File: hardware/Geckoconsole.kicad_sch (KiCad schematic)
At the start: 61 parts, among them J1 Conn_01x08_Male, J11 Conn_01x06_Male, J31 Conn_01x07_Female, J50 USB-C, J51 Conn_01x06_Male, J70 I²C, J81 Conn_01x07, Q51 S8050, Q52 S8050, SW2 Reset, SW41 Rotary_Encoder_Switch, U1 ESP32-WROOM-32, U101 AMS1117-3.3, U2 CP2102

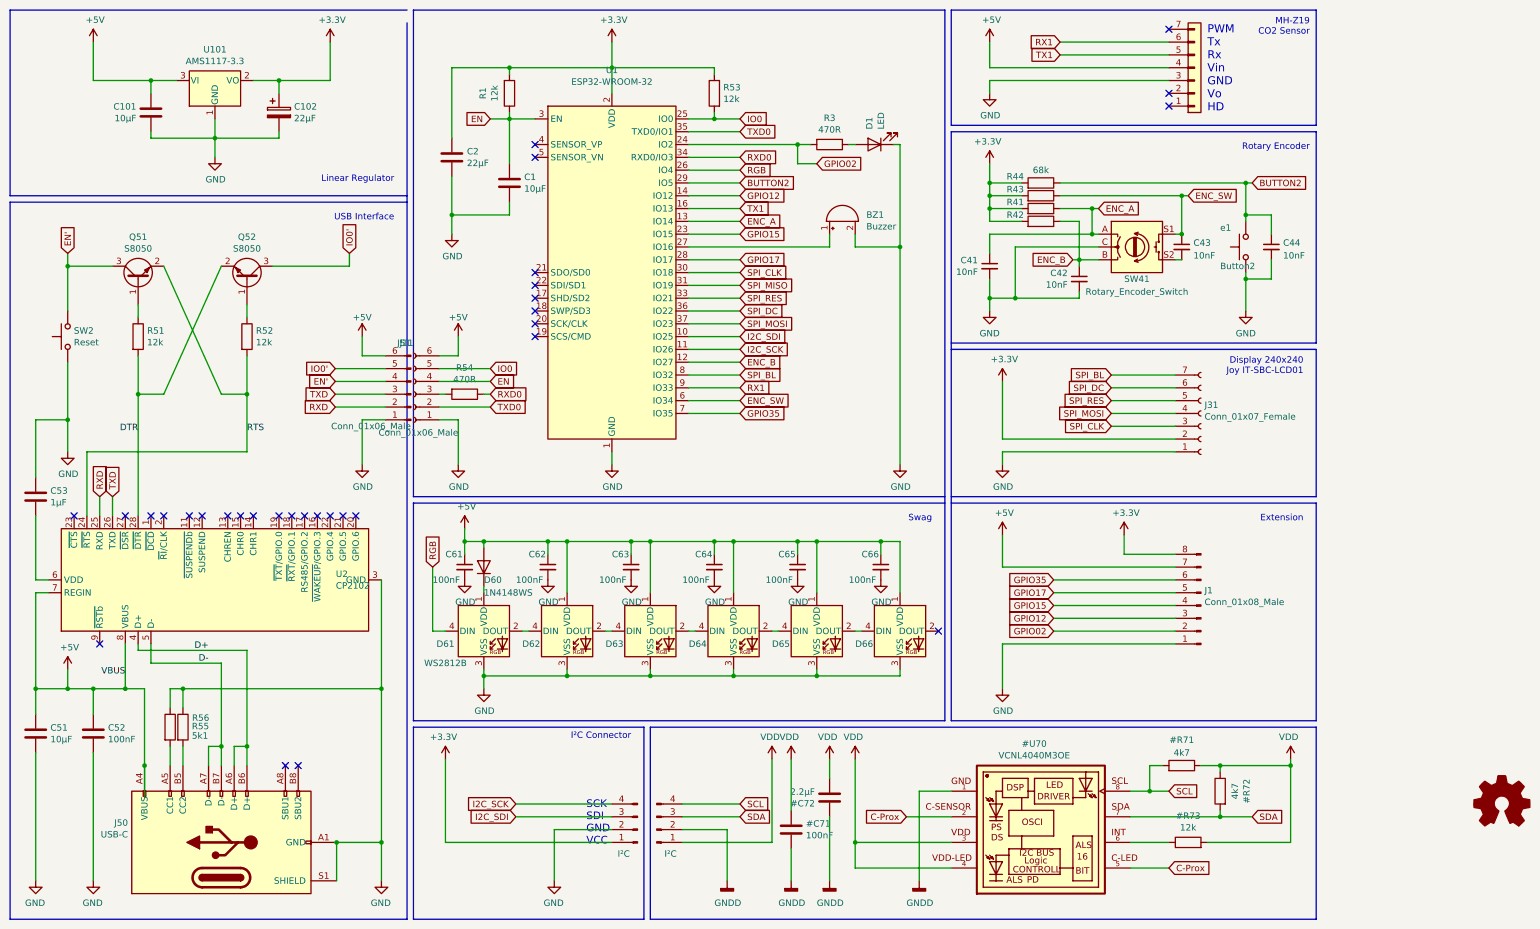
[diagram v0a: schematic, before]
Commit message: Hardware Console: Route PCB, Pannelize
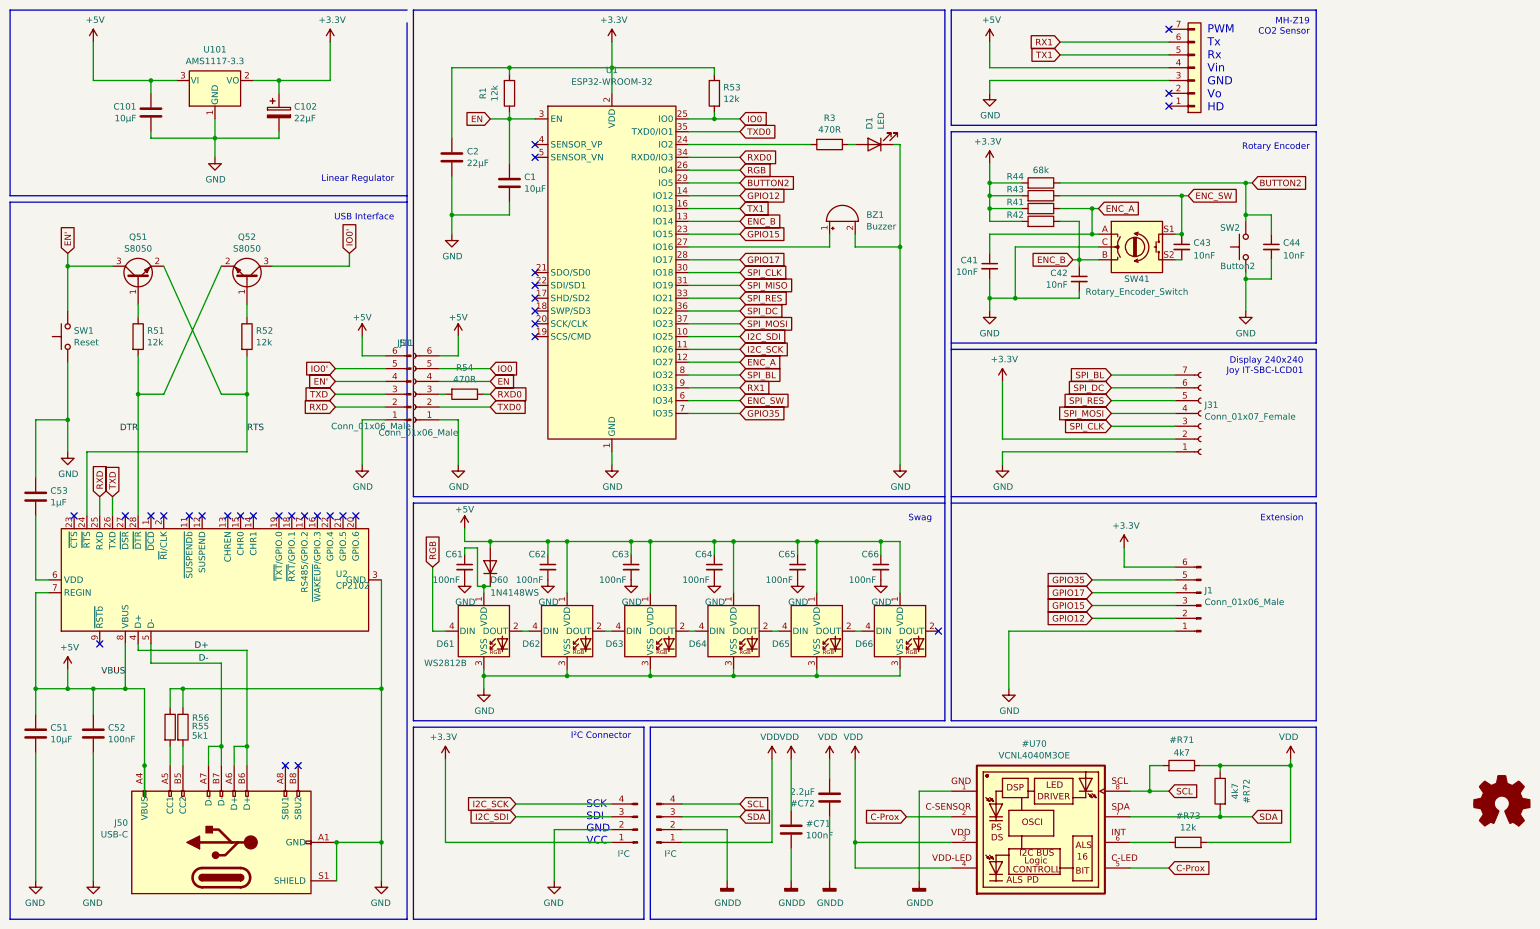
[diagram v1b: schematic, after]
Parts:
- J1: value Conn_01x08_Male -> Conn_01x06_Male; footprint Connector_PinHeader_2.54mm:PinHeader_2x04_P2.54mm_Vertical -> Connector_PinHeader_2.54mm:PinHeader_2x03_P2.54mm_Vertical; symbol Connector:Conn_01x08_Male -> Connector:Conn_01x06_Male
- renumbered SW2 to SW1, e1 to SW2
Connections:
- net +3V3: now also J1.6 (Pin_6); no longer J1.8 (Pin_8)
- net +5V: no longer C61.1, J1.7 (Pin_7)
- net ENC_A: now also U1.12 (IO27); no longer U1.13 (IO14)
- net ENC_B: now also U1.13 (IO14); no longer U1.12 (IO27)
- net GPIO12: now also J1.2 (Pin_2); no longer J1.3 (Pin_3)
- net GPIO15: now also J1.3 (Pin_3); no longer J1.4 (Pin_4)
- net GPIO17: now also J1.4 (Pin_4); no longer J1.5 (Pin_5)
- net GPIO35: now also J1.5 (Pin_5); no longer J1.6 (Pin_6)
- net at D60.1 (K), D61.1 (VDD): now also C61.1
- net GPIO02: no longer names the net of R3.2, U1.24 (IO2)
- net GPIO02: no longer J1.2 (Pin_2)
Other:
- moved on the sheet: D60
